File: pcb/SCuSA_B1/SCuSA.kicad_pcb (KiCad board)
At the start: 2 copper layers, 51 x 42 mm, 71 parts, among them J101 USB4135-GF-A, J102 JST_S2B-PH-K-x, J103 Binding_Post_PKI_10_A_Au, J104 Binding_Post_PKI_10_A_Au, J105 SMA_Straight_Jack_Female, J107 77311-118-02LF, J108 77311-118-02LF, Q101 DMN2041LSD, SW101 JS202011CQN, SW102 JS202011CQN, U101 MCP73832T-2ACI/OT, U102 BQ29700DSER, U103 TLV803EA30DBZR, U105 AD8418AWBRZ, U106 AD8655ARZ, U111 LM2775DSG

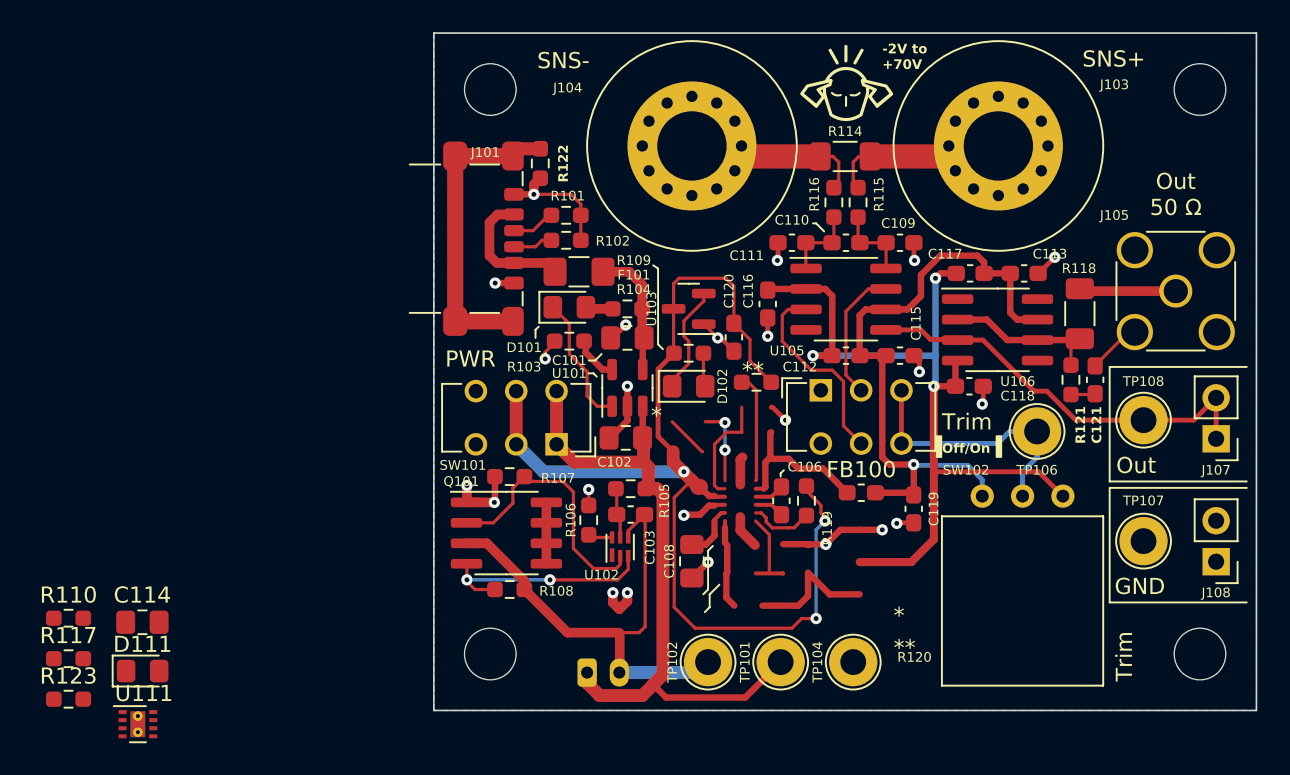
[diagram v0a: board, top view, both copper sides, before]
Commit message: Change voltage supervisor
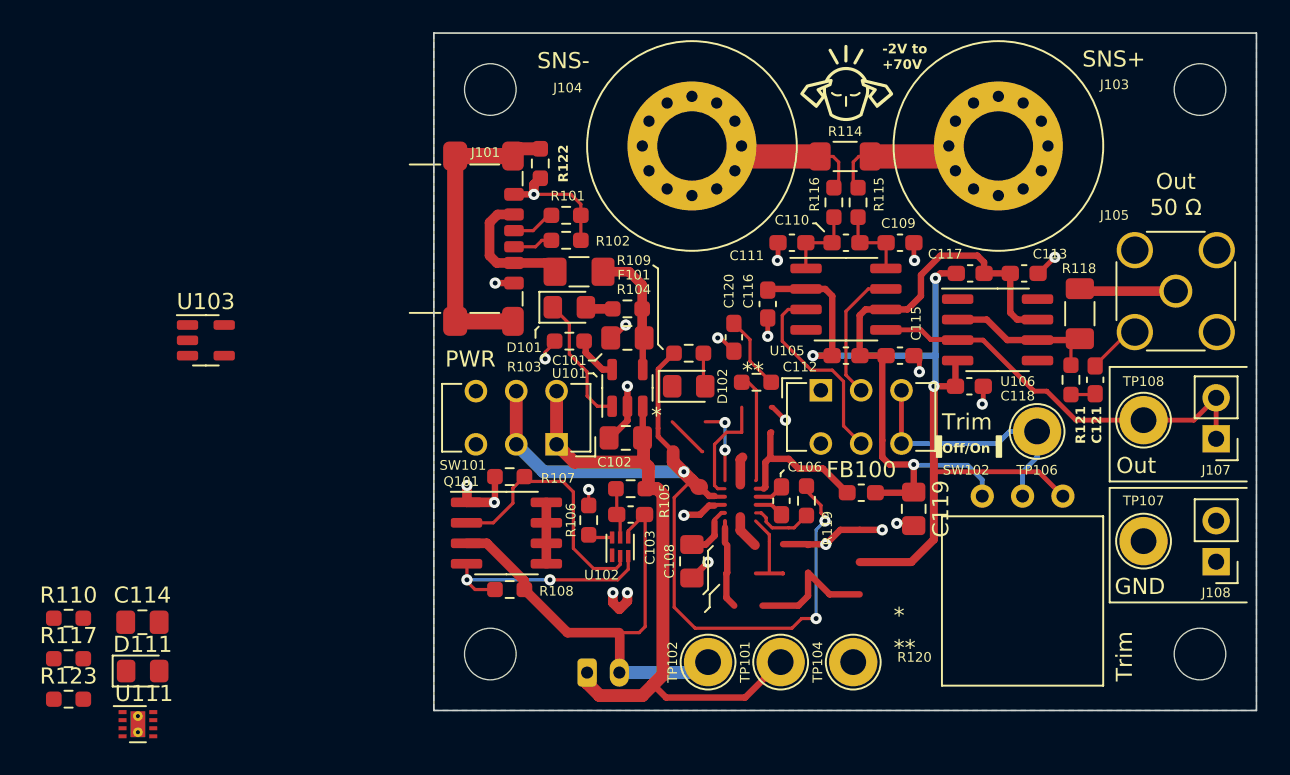
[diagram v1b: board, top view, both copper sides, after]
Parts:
- C119: value 1uF,16V,X7R,0603 -> 4.7uF,25V,X7R,0805; footprint Capacitor_SMD:C_0603_1608Metric_Pad1.08x0.95mm_HandSolder -> Capacitor_SMD:C_0805_2012Metric_Pad1.18x1.45mm_HandSolder
- U103: value TLV803EA30DBZR -> BD4836G-xx; footprint Package_TO_SOT_SMD:SOT-23 -> Package_TO_SOT_SMD:SOT-23-5
- moved U103 30.0 mm to (97.9, 81.0), turned to 0 degrees
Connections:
- net +3V3 renamed +5V
- U103 pad 1: GND -> Net-(D102-K)
- U103 pad 2: Net-(D102-K) -> /VBat_SW
- U103 pad 3: /VBat_SW -> GND
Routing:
- net /VBat_SW: track 68.4 -> 57.7 mm
- net Net-(D102-K): track 6.81 -> 0.38 mm
- net GND: track 103.7 -> 102.5 mm

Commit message: Edit PCB layout
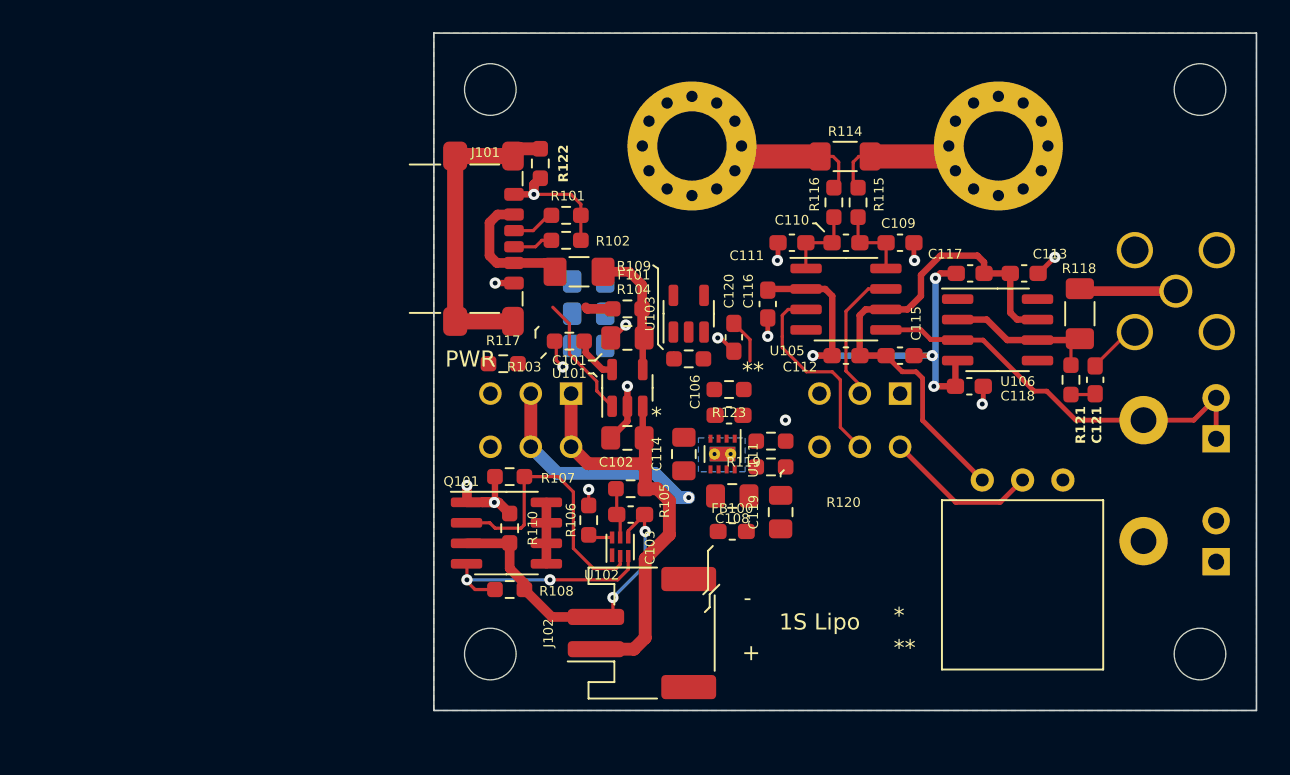
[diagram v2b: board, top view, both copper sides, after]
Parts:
- removed TP101: TestPoint_5010_Red, TestPoint:TestPoint_Loop_D2.60mm_Drill1.6mm_Beaded
- removed TP102, TP104: TestPoint_5011_Black, TestPoint:TestPoint_Loop_D2.60mm_Drill1.6mm_Beaded
- removed TP106: TestPoint_5012_White, TestPoint:TestPoint_Loop_D2.60mm_Drill1.6mm_Beaded
- D101, D102, D111, G***, J103, J104, J105, J107, J108, SW101, SW102, TP107, TP108: moved to B.Cu
- J102: value JST_S2B-PH-K-x -> JST_S2B-PH-SM4-x; footprint Connector_JST:JST_PH_S2B-PH-K_1x02_P2.00mm_Horizontal -> Connector_User:JST_PH_S2B-PH-SM4-TB_1x02-1MP_P2.00mm_Horizontal; moved to F.Cu
- moved R123 45.2 mm to (130.3, 84.1), turned to 180 degrees
- moved U111 39.9 mm to (129.9, 88.1), turned to -90 degrees
- moved C114 35.2 mm to (127.5, 88.1), turned to 90 degrees
- moved D111 34.2 mm to (121.6, 81.4), turned to 180 degrees
- moved R117 32.6 mm to (116.3, 82.5)
- moved U103 30.0 mm to (127.8, 79.4), turned to 90 degrees
- moved R110 27.9 mm to (116.7, 92.7), turned to -90 degrees
- moved FB100 8.35 mm to (130.5, 92.9)
- moved C119 8.25 mm to (133.5, 91.7), turned to 90 degrees
- moved D102 7.66 mm to (121.6, 79.4), turned to 180 degrees
- moved C106 6.22 mm to (130.3, 85.7), turned to 0 degrees
- moved G*** 6.10 mm to (137.4, 71.4), turned to 180 degrees
- moved R120 5.33 mm to (132.9, 88.9)
- moved SW102 4.92 mm to (140.9, 84.3), turned to 180 degrees
- moved C108 4.76 mm to (130.5, 90.7), turned to 0 degrees
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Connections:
- RV101 pad 2: Net-(SW102A-C) -> Net-(SW102A-A)
- SW102 pad 1: GND -> Net-(SW102A-A)
- SW102 pad 3: Net-(SW102A-C) -> GND
- SW102 pad 4: GND -> Net-(SW102A-A)
- SW102 pad 6: Net-(SW102A-C) -> GND
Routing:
- net /VBat_SW: track 57.7 -> 17.4 mm, vias 3 -> 1
- net GND: track 102.5 -> 62.5 mm, vias 26 -> 19
- net (no net): track 33.4 -> 0.00 mm, vias 2 -> 0
- net Net-(SW102A-C): track 16.4 -> 0.00 mm
- net /VBat: track 42.2 -> 27.7 mm
- net Net-(U111-VOUT): track 13.3 -> 0.00 mm
- net Net-(U111-PFM): track 10.7 -> 0.00 mm
- net Net-(SW102A-A): track 0.00 -> 9.60 mm
- net /Cell-: track 31.0 -> 22.2 mm, vias 0 -> 2
- net +5V: track 39.4 -> 31.9 mm, vias 1 -> 0
- net Net-(D102-A): track 2.10 -> 0.00 mm
- net Net-(U111-C1-): track 1.85 -> 0.00 mm
- net Net-(U111-C1+): track 1.85 -> 0.00 mm
- net Net-(Q101A-G1): track 16.3 -> 17.8 mm
- net Net-(D101-K): track 8.19 -> 7.66 mm
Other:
- board text added: "Charging"
- board text added: "Low Bat"
- board text added: "Max. -2V to +70V"
- board text added: "Power"
- board text added: "Power On/Off"
- board text added: "SCuSA Scope Current Sense Amplifier Rev B1, by fl0m0"
- board text added: "Trim +←→-"
- board text added: "Trim On/Off"
- board text removed: "-2V to +70V"
- board text removed: "Off/On"
- board text removed: "Scope Current Sense Amplifier SCuSA - Rev B1 by fl0m0"
- board text removed: "Trim"
